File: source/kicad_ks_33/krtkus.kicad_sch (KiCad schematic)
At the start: 123 parts, among them SW1 Push, SW10 Push, SW11 Push, SW12 Push, SW14 Push, SW15 Push, SW16 Push, SW17 Push, SW18 Push, SW2 Push, SW20 Push, SW21 Push, SW22 Push, SW23 Push, SW24 Push, SW26 Push, SW27 Push, SW28 Push, SW29 Push, SW3 Push, SW30 Push, SW32 Push, SW33 Push, SW34 Push, SW35 Push, SW38 Push, SW39 Push, SW4 Push, SW40 Push, SW41 Push, SW42 Push, SW44 Push, SW45 Push, SW46 Push, SW47 Push, SW48 Push, SW5 Push, SW50 Push, SW51 Push, SW52 Push, SW53 Push, SW54 Push, SW56 Push, SW57 Push, SW58 Push, SW59 Push, SW6 Push, SW60 Push, SW62 Push, SW63 Push, SW64 Push, SW65 Push, SW66 Push, SW67 Push, SW68 Push, SW69 Push, SW70 Push, SW71 Push, SW72 Push, SW8 Push, SW9 Push, U1 Arduino_Pro_Micro

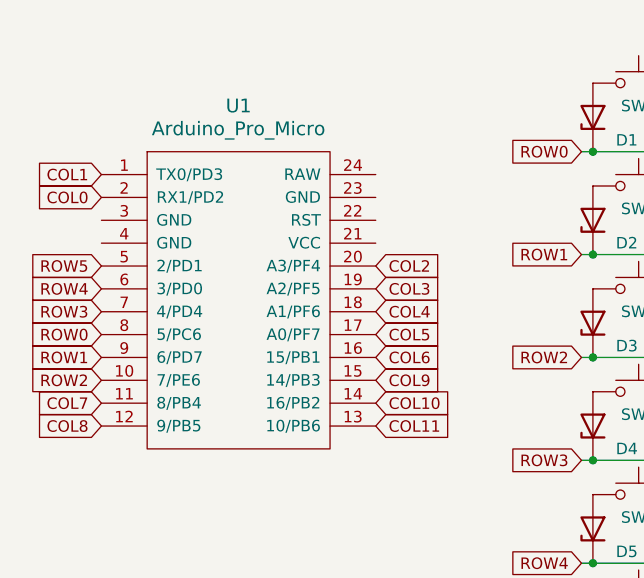
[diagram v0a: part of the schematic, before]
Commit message: unification
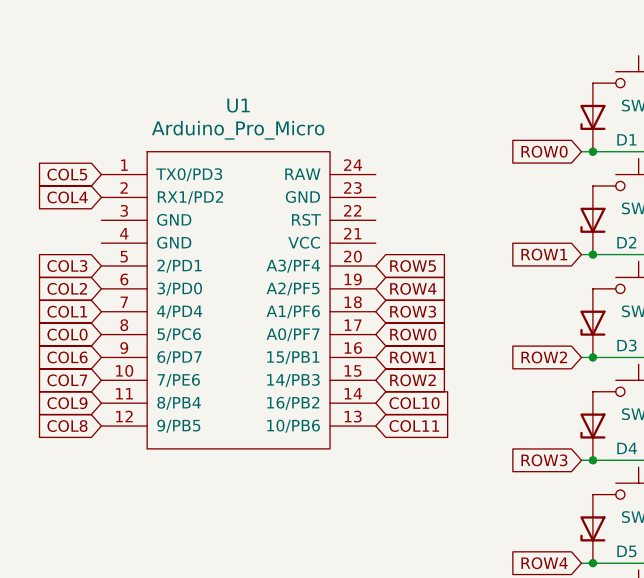
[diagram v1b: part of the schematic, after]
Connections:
- net COL0: now also U1.8 (5/PC6); no longer U1.2 (RX1/PD2)
- net COL1: now also U1.7 (4/PD4); no longer U1.1 (TX0/PD3)
- net COL2: now also U1.6 (3/PD0); no longer U1.20 (A3/PF4)
- net COL3: now also U1.5 (2/PD1); no longer U1.19 (A2/PF5)
- net COL4: now also U1.2 (RX1/PD2); no longer U1.18 (A1/PF6)
- net COL5: now also U1.1 (TX0/PD3); no longer U1.17 (A0/PF7)
- net COL6: now also U1.9 (6/PD7); no longer U1.16 (15/PB1)
- net COL7: now also U1.10 (7/PE6); no longer U1.11 (8/PB4)
- net COL9: now also U1.11 (8/PB4); no longer U1.15 (14/PB3)
- net ROW0: now also U1.17 (A0/PF7); no longer U1.8 (5/PC6)
- net ROW1: now also U1.16 (15/PB1); no longer U1.9 (6/PD7)
- net ROW2: now also U1.15 (14/PB3); no longer U1.10 (7/PE6)
- net ROW3: now also U1.18 (A1/PF6); no longer U1.7 (4/PD4)
- net ROW4: now also U1.19 (A2/PF5); no longer U1.6 (3/PD0)
- net ROW5: now also U1.20 (A3/PF4); no longer U1.5 (2/PD1)

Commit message: ks-33 footprint tweaks
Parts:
- SW1, SW10, SW11, SW12, SW14, SW15, SW16, SW17, SW18, SW2, SW20, SW21, SW22, SW23, SW24, SW26, SW27, SW28, SW29, SW3, SW30, SW32, SW33, SW34, SW35, SW38, SW39, SW4, SW40, SW41, SW42, SW44, SW45, SW46, SW47, SW48, SW5, SW50, SW51, SW52, SW53, SW54, SW56, SW57, SW58, SW59, SW6, SW60, SW62, SW63, SW64, SW65, SW66, SW67, SW68, SW69, SW70, SW71, SW72, SW8, SW9: footprint Gateron_KS33_Solderable:Gateron-KS33-Solderable-1U -> Gateron_KS33_Solderable:Gateron-KS33-Solderable-1U-Tight
